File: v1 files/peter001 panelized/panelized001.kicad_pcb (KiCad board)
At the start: 2 copper layers, 98.7 x 98.3 mm, 20 parts

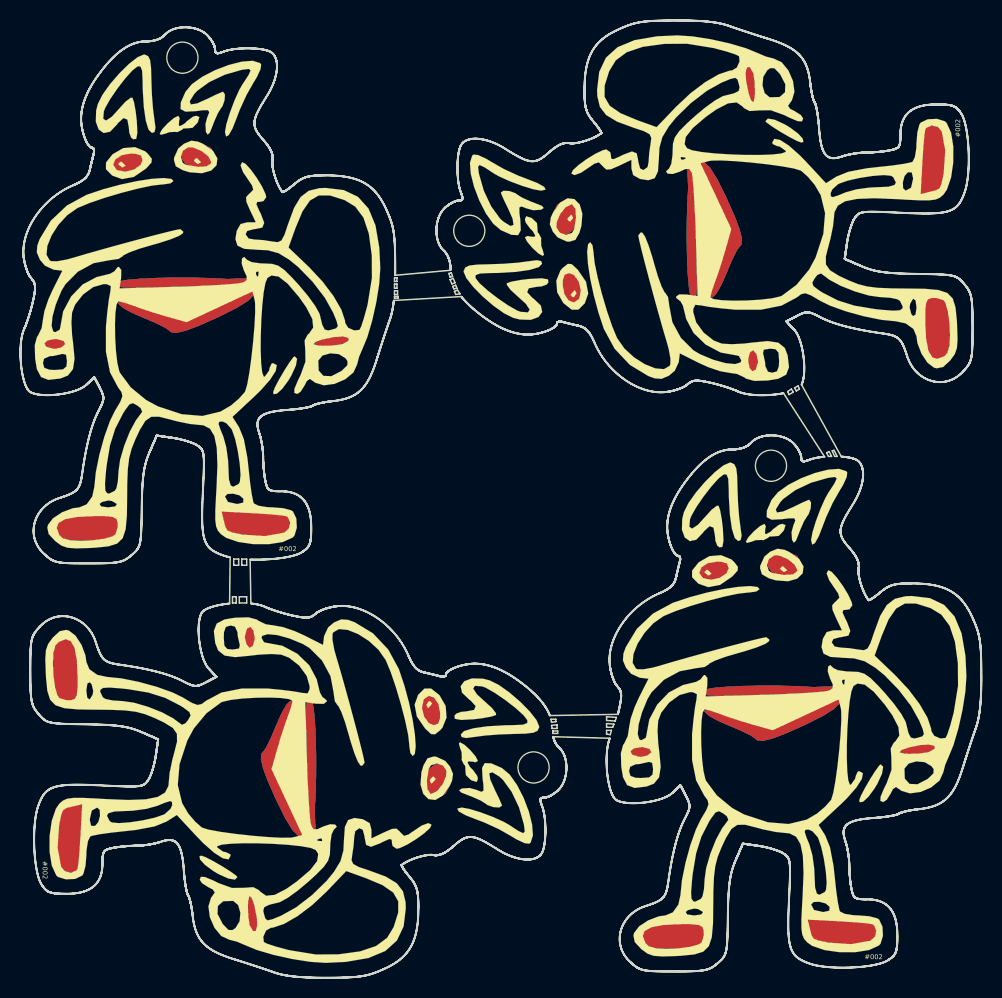
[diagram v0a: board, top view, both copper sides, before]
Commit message: updated panelzing
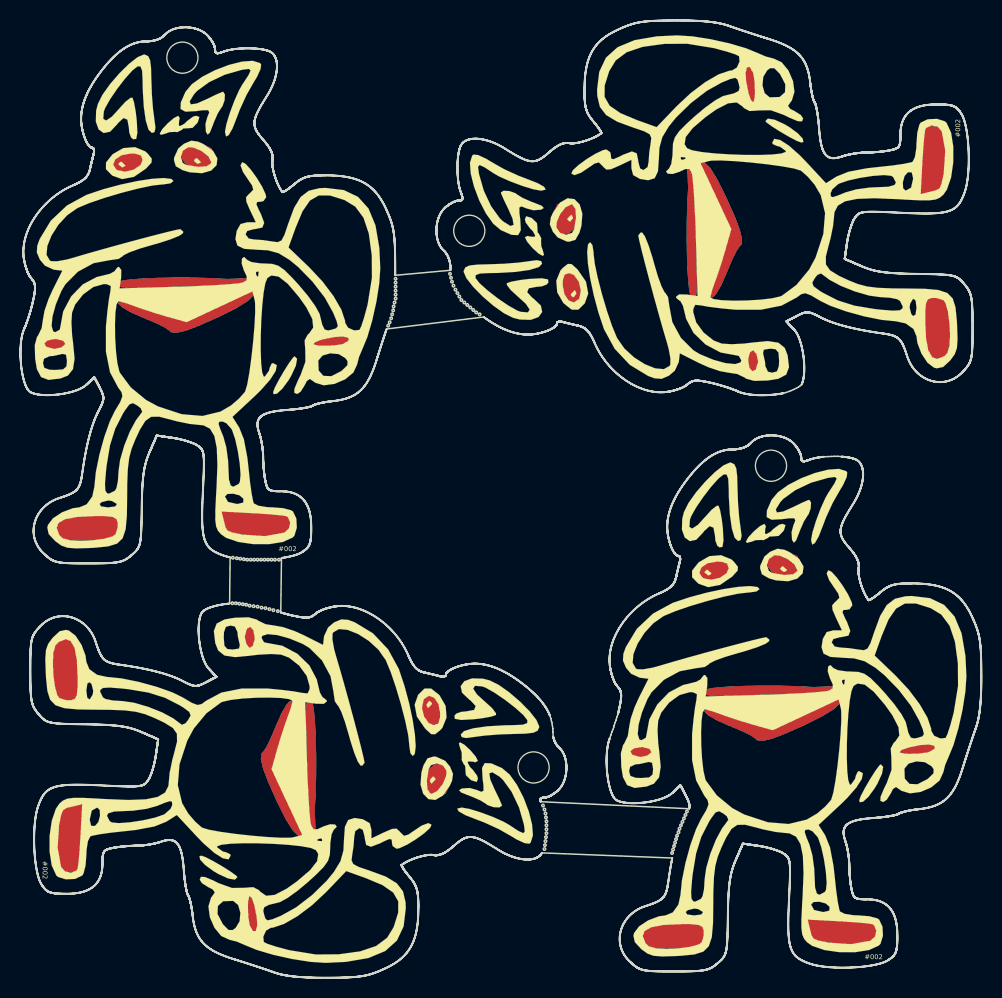
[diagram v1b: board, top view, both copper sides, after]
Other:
- outline, holes or cut-outs redrawn
